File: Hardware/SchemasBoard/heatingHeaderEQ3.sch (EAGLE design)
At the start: 27 parts, among them IC1 LNK304, IC2 MCP1703DB, IC4 DS1820, K1 FRS1B, T1 BC846

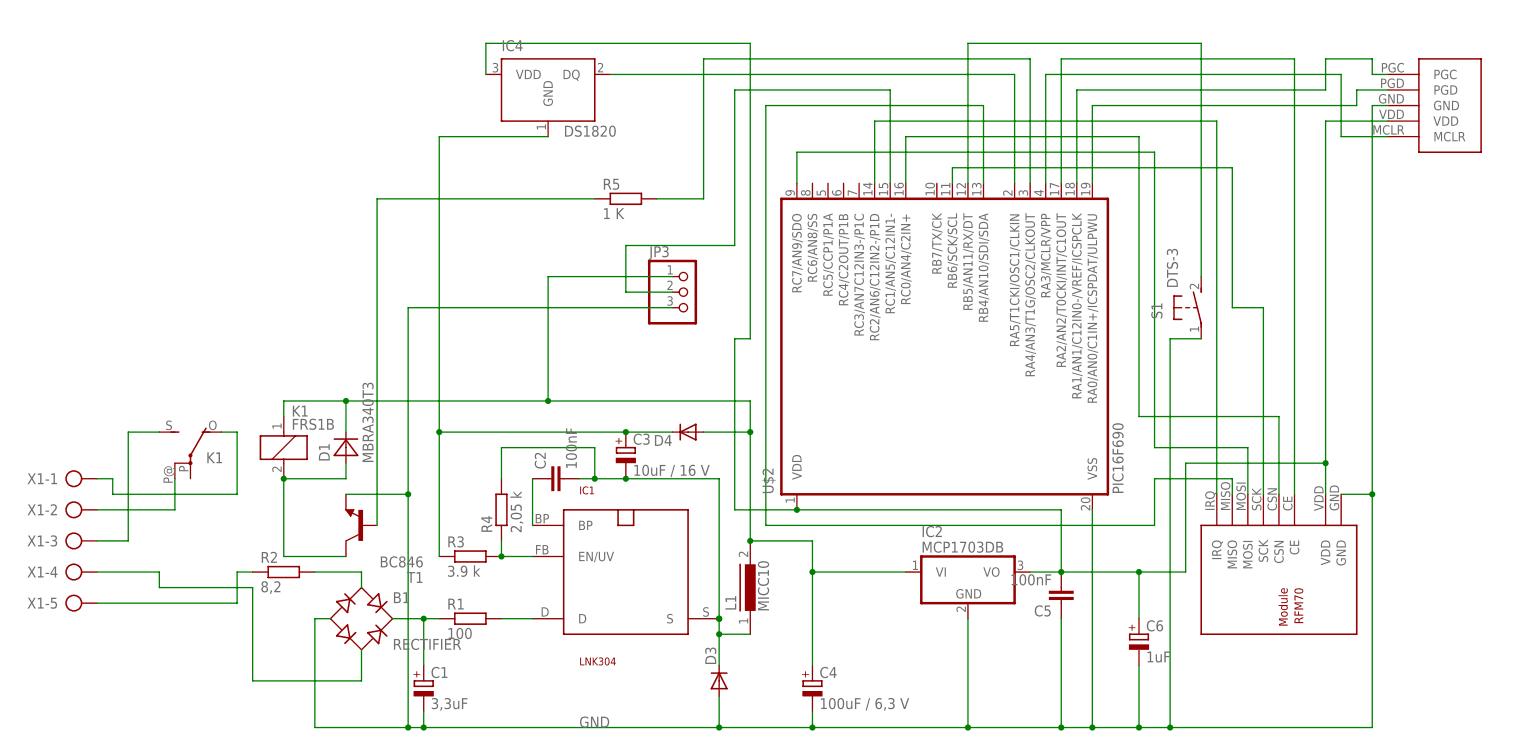
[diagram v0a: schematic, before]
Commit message: a
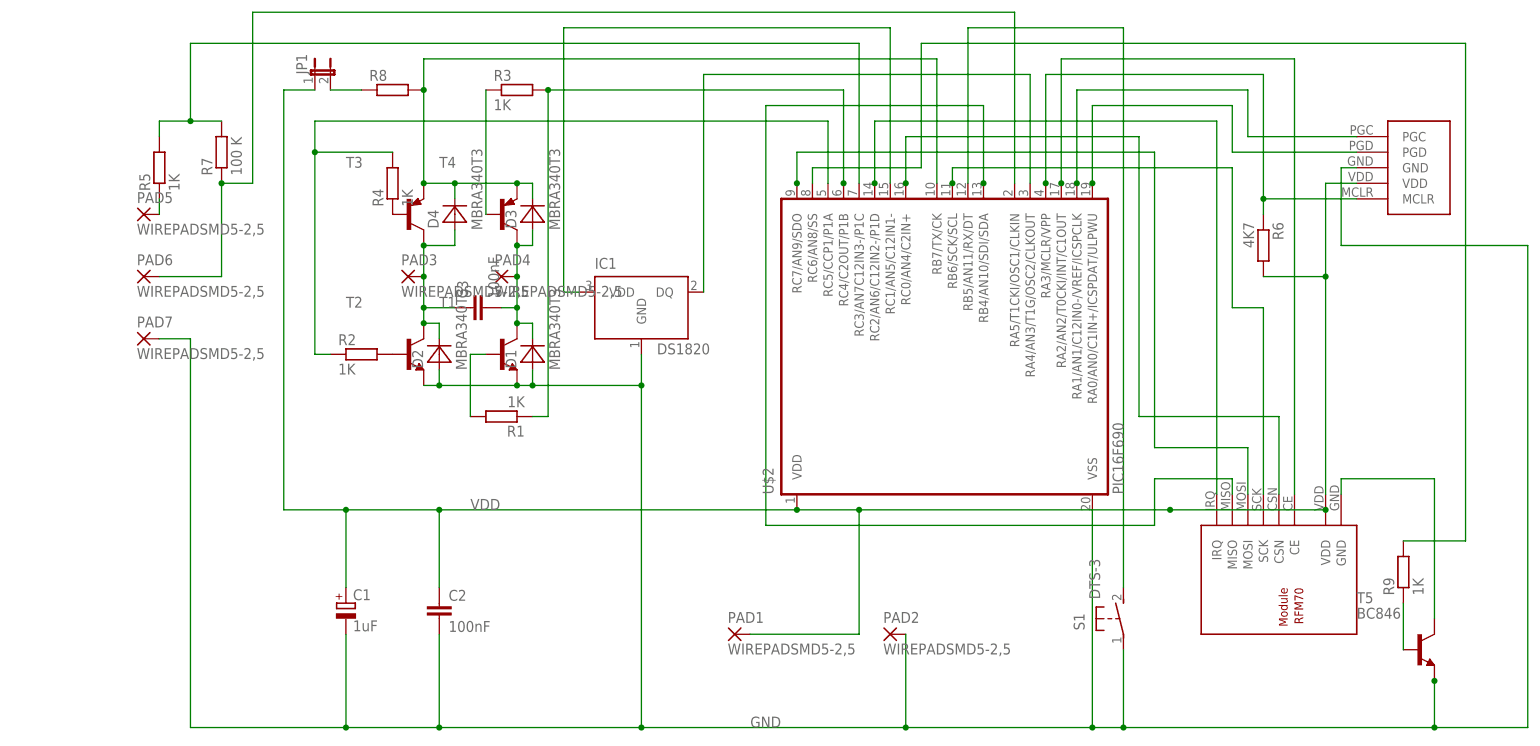
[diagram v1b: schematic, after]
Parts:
- removed B1: RECTIFIER, rectifier:RECTIFIER-S40
- removed C4: 100uF / 6,3 V, resistor:CPOL-EUE2.5-5
- removed C5: 100nF, resistor:C-EUC2012
- removed C6: 1uF, resistor:CPOL-EUSMCA
- removed IC2: MCP1703DB, linear:MCP1703DB
- removed IC4: DS1820, ds1820:DS1820
- removed JP3: (no value), pinhead:PINHD-1X3
- removed K1: FRS1B, relay:FRS1B
- removed L1: MICC10, inductors:MICC10
- removed X1: (no value), con-ptr500:AK500/5
- added D2: MBRA340T3, diode:MBRA340T3
- added JP1: (no value), jumper:JP1E
- added PAD1, PAD2, PAD3, PAD4, PAD5, PAD6, PAD7: WIREPADSMD5-2,5, wirepad:WIREPADSMD5-2,5
- added R6: 4K7, resistor:R-EU_R1206W
- added R7: 100 K, resistor:R-EU_R1206
- added R8: (no value), resistor:R-EU_R2512W
- added R9: 1K, resistor:R-EU_R1206
- added T2: (no value), transistor:BC817-40-NPN-SOT23-BEC
- added T3, T4: (no value), transistor:BC807-16-PNP-SOT23-BEC
- added T5: BC846, transistor:BC846
- C1: value 3,3uF -> 1uF; device resistor:CPOL-EUE5-10.5 -> resistor:CPOL-EUSMCA
- C3: value 10uF / 16 V -> 100nF; device resistor:CPOL-EUE2.5-5 -> resistor:C-EUC2012
- D3, D4: value (none) -> MBRA340T3; device diode:DIODE-DO214AA -> diode:MBRA340T3
- IC1: value LNK304 -> DS1820; device powerint:SO-8C -> ds1820:DS1820
- R1: value 100 -> 1K; device resistor:R-EU_R2512W -> resistor:R-EU_R1206
- R2: value 8,2 -> 1K; device resistor:R-EU_R2512W -> resistor:R-EU_R1206
- R3: value 3.9 k -> 1K; device resistor:R-EU_M2012 -> resistor:R-EU_R1206
- R4: value 2,05 k -> 1K; device resistor:R-EU_M2012 -> resistor:R-EU_R1206
- R5: value 1 K -> 1K; device resistor:R-EU_M2012 -> resistor:R-EU_R1206
- T1: value BC846 -> (none); device transistor:BC846 -> transistor:BC817-40-NPN-SOT23-BEC
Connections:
- removed net N$10 (its old number): C2.1, IC1.BP
- removed net N$17: C5.2, C6.+, IC2.VO, IC4.VDD, U$1.VDD, U$2.VDD, U$3.VDD
- removed net N$26: C4.+, D1.C, D4.A, IC2.VI, JP3.1, K11.1, L1.2
- removed net N$32: JP3.2, U$2.RC1/AN5/C12IN1-
- removed net N$35: R5.2, U$2.RA4/AN3/T1G/OSC2/CLKOUT
- removed net N$36: R2.1, X1-5.KL
- removed net N$6 (its old number): IC4.DQ, U$2.RA5/T1CKI/OSC1/CLKIN
- new net N$12: R5.2, R7.2, U$2.RC3/AN7C12IN3-/P1C
- new net N$27: R3.1, T4.B
- new net N$28: T5.C, U$1.GND
- new net N$30: R1.1, R3.2, U$2.RC4/C2OUT/P1B
- new net N$31: R2.1, R4.2, U$2.RC5/CCP1/P1A
- new net N$5: R9.1, T5.B
- new net VDD: C1.+, C2.1, JP1.1, PAD1.P, R6.2, U$1.VDD, U$2.VDD, U$3.VDD
- net GND: now also C2.2, D1.A, D2.A, IC1.GND, PAD2.P, PAD7.P, T2.E, T5.E; no longer B1.-, C4.-, C5.1, C6.-, D3.A, IC2.GND, JP3.3, U$1.GND
- net N$1: now also IC1.DQ, U$2.RA4/AN3/T1G/OSC2/CLKOUT; no longer IC1.D, R1.2
- net N$11: now also R9.2, U$2.RC6/AN8/SS; no longer IC1.EN/UV, R3.2, R4.1
- net N$13: now also R2.2, T2.B; no longer C2.2, C3.-, D3.C, IC1.S, L1.1, R4.2
- net N$14: now also R4.1, T3.B; no longer D1.A, K11.2, T1.C
- net N$15: now also D3.C, D4.C, R8.2, T3.E, T4.E, U$2.RB7/TX/CK; no longer R5.1, T1.B
- net N$2: now also JP1.2, R8.1; no longer B1.+, C1.+, R1.1
- net N$24: now also R1.2, T1.B; no longer K12.O, X1-1.KL
- net N$25: now also R6.1
- net N$3: now also IC1.VDD, U$2.RC1/AN5/C12IN1-; no longer B1.AC1, R2.2
- net N$4: now also PAD5.P, R5.1; no longer B1.AC2, X1-4.KL
- net N$7: now also C3.1, D2.C, D4.A, PAD3.P, T2.C, T3.C; no longer K12.P@1, X1-2.KL
- net N$8: now also C3.2, D1.C, D3.A, PAD4.P, T1.C, T4.C; no longer K12.S, X1-3.KL
- net N$9: now also PAD6.P, R7.1, U$2.RA5/T1CKI/OSC1/CLKIN; no longer C3.+, D4.C, IC4.GND, R3.1
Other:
- moved on the sheet: C1, C2, D1, R1, R2, R3, R4, R5, S1, T1

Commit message: dfg
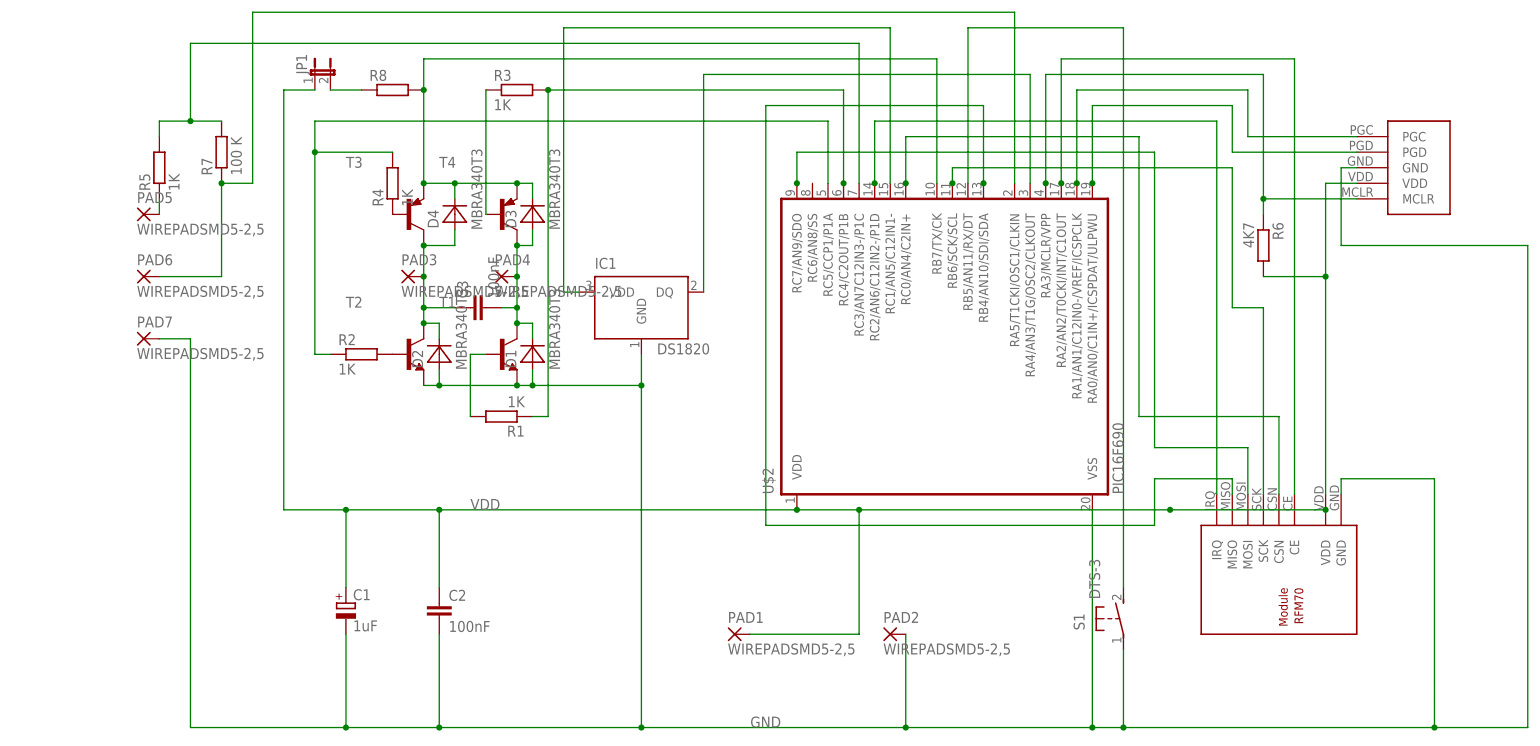
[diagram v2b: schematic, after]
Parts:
- removed R9: 1K, resistor:R-EU_R1206
- removed T5: BC846, transistor:BC846
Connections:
- removed net N$11: R9.2, U$2.RC6/AN8/SS
- removed net N$28: T5.C, U$1.GND
- removed net N$5: R9.1, T5.B
- net GND: now also U$1.GND; no longer T5.E
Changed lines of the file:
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@@
 <part name="R6" library="resistor" deviceset="R-EU_" device="R1206W" value="4K7"/>
 <part name="U$3" library="rfm70" deviceset="PROGRAMMINGHEADER" device="" technology="DIP"/>
-<part name="T5" library="transistor" deviceset="BC846" device=""/>
-<part name="R9" library="resistor" deviceset="R-EU_" device="R1206" value="1K"/>
 <part name="C3" library="resistor" deviceset="C-EU" device="C2012" value="100nF"/>
 </parts>
@@
 <instance part="R6" gate="G$1" x="160.02" y="109.22" rot="R270"/>
 <instance part="U$3" gate="G$1" x="185.42" y="121.92"/>
-<instance part="T5" gate="G$1" x="185.42" y="43.18"/>
-<instance part="R9" gate="G$1" x="182.88" y="55.88" rot="R90"/>
 <instance part="C3" gate="G$1" x="30.48" y="99.06" rot="R90"/>
 </instances>
@@
 <wire x1="132.08" y1="66.04" x2="132.08" y2="30.48" width="0.1524" layer="91"/>
 <pinref part="IC1" gate="G$1" pin="GND"/>
-<wire x1="187.96" y1="38.1" x2="187.96" y2="30.48" width="0.1524" layer="91"/>
+<wire x1="187.96" y1="38.1" x2="187.96" y2="35.56" width="0.1524" layer="91"/>
+<wire x1="187.96" y1="35.56" x2="187.96" y2="30.48" width="0.1524" layer="91"/>
 <wire x1="58.42" y1="91.44" x2="58.42" y2="86.36" width="0.1524" layer="91"/>
 <wire x1="58.42" y1="86.36" x2="58.42" y2="30.48" width="0.1524" layer="91"/>
@@
 <wire x1="203.2" y1="30.48" x2="187.96" y2="30.48" width="0.1524" layer="91"/>
 <junction x="187.96" y="30.48"/>
-<pinref part="T5" gate="G$1" pin="E"/>
-<junction x="187.96" y="38.1"/>
+<pinref part="U$1" gate="G$1" pin="GND"/>
+<wire x1="172.72" y1="71.12" x2="172.72" y2="68.58" width="0.1524" layer="91"/>
+<wire x1="187.96" y1="38.1" x2="187.96" y2="71.12" width="0.1524" layer="91"/>
+<wire x1="187.96" y1="71.12" x2="172.72" y2="71.12" width="0.1524" layer="91"/>
 </segment>
 </net>
@@
 </segment>
 </net>
-<net name="N$5" class="0">
-<segment>
-<pinref part="R9" gate="G$1" pin="1"/>
-<pinref part="T5" gate="G$1" pin="B"/>
-<wire x1="182.88" y1="50.8" x2="182.88" y2="43.18" width="0.1524" layer="91"/>
-</segment>
-</net>
-<net name="N$11" class="0">
-<segment>
-<pinref part="R9" gate="G$1" pin="2"/>
-<wire x1="182.88" y1="60.96" x2="193.04" y2="60.96" width="0.1524" layer="91"/>
-<wire x1="193.04" y1="60.96" x2="193.04" y2="142.24" width="0.1524" layer="91"/>
-<wire x1="193.04" y1="142.24" x2="104.14" y2="142.24" width="0.1524" layer="91"/>
-<wire x1="104.14" y1="142.24" x2="104.14" y2="121.92" width="0.1524" layer="91"/>
-<pinref part="U$2" gate="G$1" pin="RC6/AN8/SS"/>
-<wire x1="104.14" y1="121.92" x2="86.36" y2="121.92" width="0.1524" layer="91"/>
-<wire x1="86.36" y1="121.92" x2="86.36" y2="119.38" width="0.1524" layer="91"/>
-</segment>
-</net>
-<net name="N$28" class="0">
-<segment>
-<pinref part="U$1" gate="G$1" pin="GND"/>
-<wire x1="172.72" y1="71.12" x2="172.72" y2="68.58" width="0.1524" layer="91"/>
-<pinref part="T5" gate="G$1" pin="C"/>
-<wire x1="187.96" y1="48.26" x2="187.96" y2="71.12" width="0.1524" layer="91"/>
-<wire x1="187.96" y1="71.12" x2="172.72" y2="71.12" width="0.1524" layer="91"/>
-</segment>
-</net>
